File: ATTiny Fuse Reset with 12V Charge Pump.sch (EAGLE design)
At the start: 62 parts, among them IC1 74HC04D, Q1 BSS138, Q2 PMV65XP, Q3 BSS138, Q4 BSS138, Q5 BSS138, Q6 BSS138, Q7 BSS138, Q8 BSS130, SW4 SWITCH_SPDT, U1 ARDUINOR3, X1 057-006-1

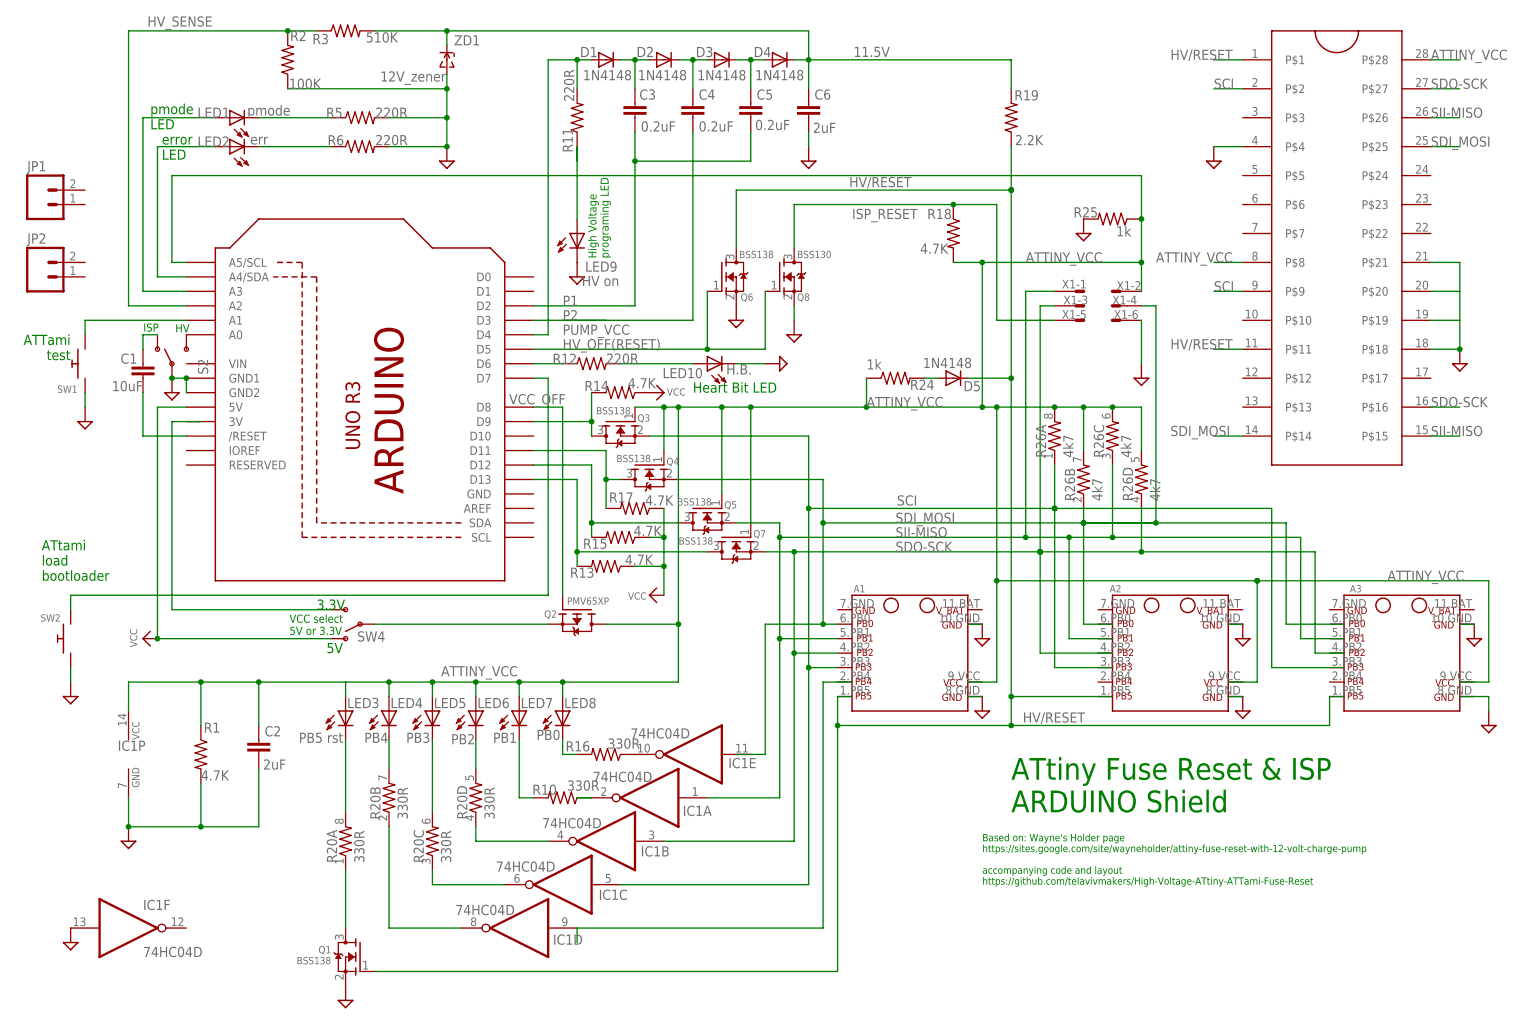
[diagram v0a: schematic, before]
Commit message: zif24 ito brd
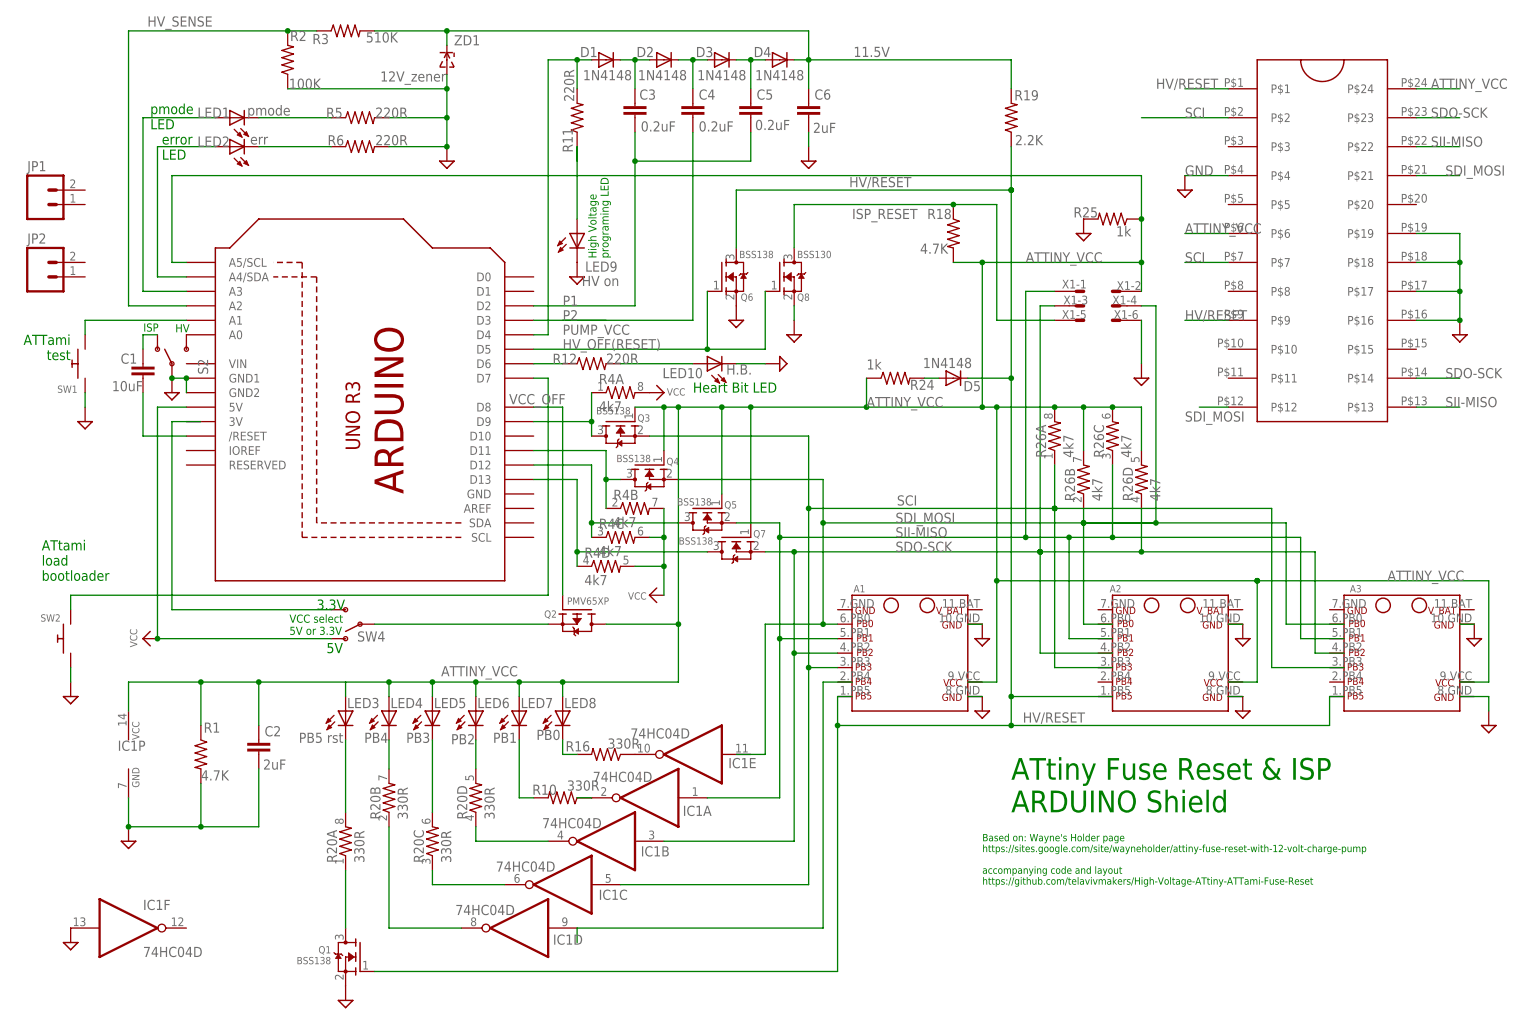
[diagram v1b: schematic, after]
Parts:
- removed R13, R14, R15, R17: 4.7K, ATtami:RESISTOR0805-RES
- removed U$1: ZIFSOCKET-28-3ZIFFSOCKET-28-3, ATTiny Fuse Reset with 12V Charge Pump:ZIFSOCKET-28-3ZIFFSOCKET-28-3
- added R4: 4k7, SparkFun-Passives:RESISTOR-ARRAY0603-ARV
- added U$2: ZIFSOCKET-24, ATTiny Fuse Reset with 12V Charge Pump:ZIFSOCKET-24
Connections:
- removed net N$50: U$1.P$20
- removed net N$51: U$1.P$19
- net ATTINY_VCC: now also U$2.P$24, U$2.P$6; no longer U$1.P$28, U$1.P$8
- net GND: now also U$2.P$16, U$2.P$17, U$2.P$18, U$2.P$19, U$2.P$4; no longer U$1.P$18, U$1.P$21, U$1.P$4
- net HV/RESET: now also U$2.P$1, U$2.P$9; no longer U$1.P$1, U$1.P$11
- net N$2: now also R4A.1; no longer R14.2
- net N$34: now also R4D.1; no longer R13.2
- net N$37: now also R4C.1; no longer R15.2
- net N$8: now also R4B.1; no longer R17.2
- net SCI: now also U$2.P$2, U$2.P$7; no longer U$1.P$2, U$1.P$9
- net SDI_MOSI: now also U$2.P$12, U$2.P$21; no longer U$1.P$14, U$1.P$25
- net SDO-SCK: now also U$2.P$14, U$2.P$23; no longer U$1.P$16, U$1.P$27
- net SII-MISO: now also U$2.P$13, U$2.P$22; no longer U$1.P$15, U$1.P$26
- net VCC: now also R4A.2, R4B.2, R4C.2, R4D.2; no longer R13.1, R14.1, R15.1, R17.1
